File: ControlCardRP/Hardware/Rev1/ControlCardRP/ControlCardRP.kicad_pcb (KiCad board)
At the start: 2 copper layers, 53.5 x 49.5 mm, 46 parts, among them J1 Conn_02x20_Top_Bottom, J2 USB_C_Receptacle_USB2.0_16P, J3 SWD, J4 JST_PK BATTERY, J5 PIN_HEADER BATTERY, SW101 BOOT0, SW102 NRST, U1 AP33772SDKZ-xx-FA02, U101 W25Q128JVS, U102 RP2354B, U103 W25Q128JVS, U2 BQ24075RGT, U3 BQ27427YZFR, U4 MP28167GQ-A-P, Y1 12MHz

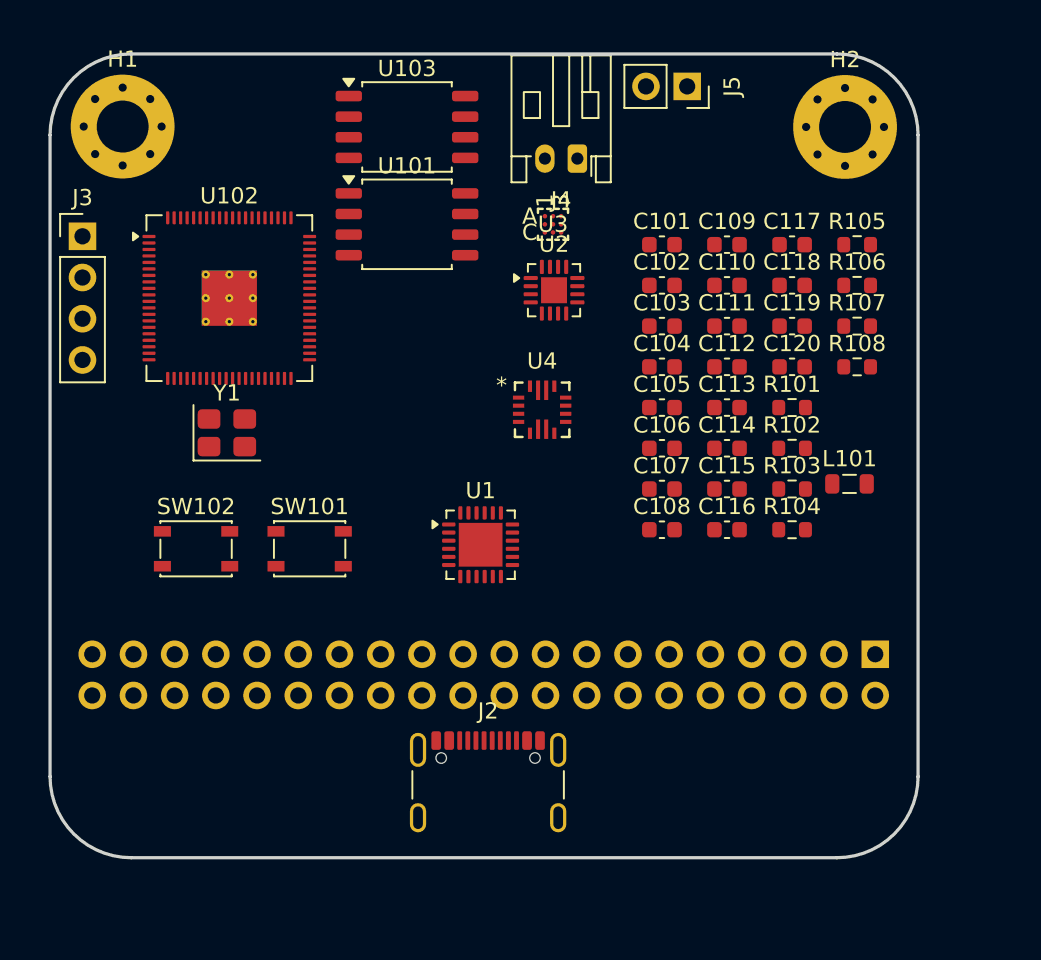
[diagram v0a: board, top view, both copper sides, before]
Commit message: A
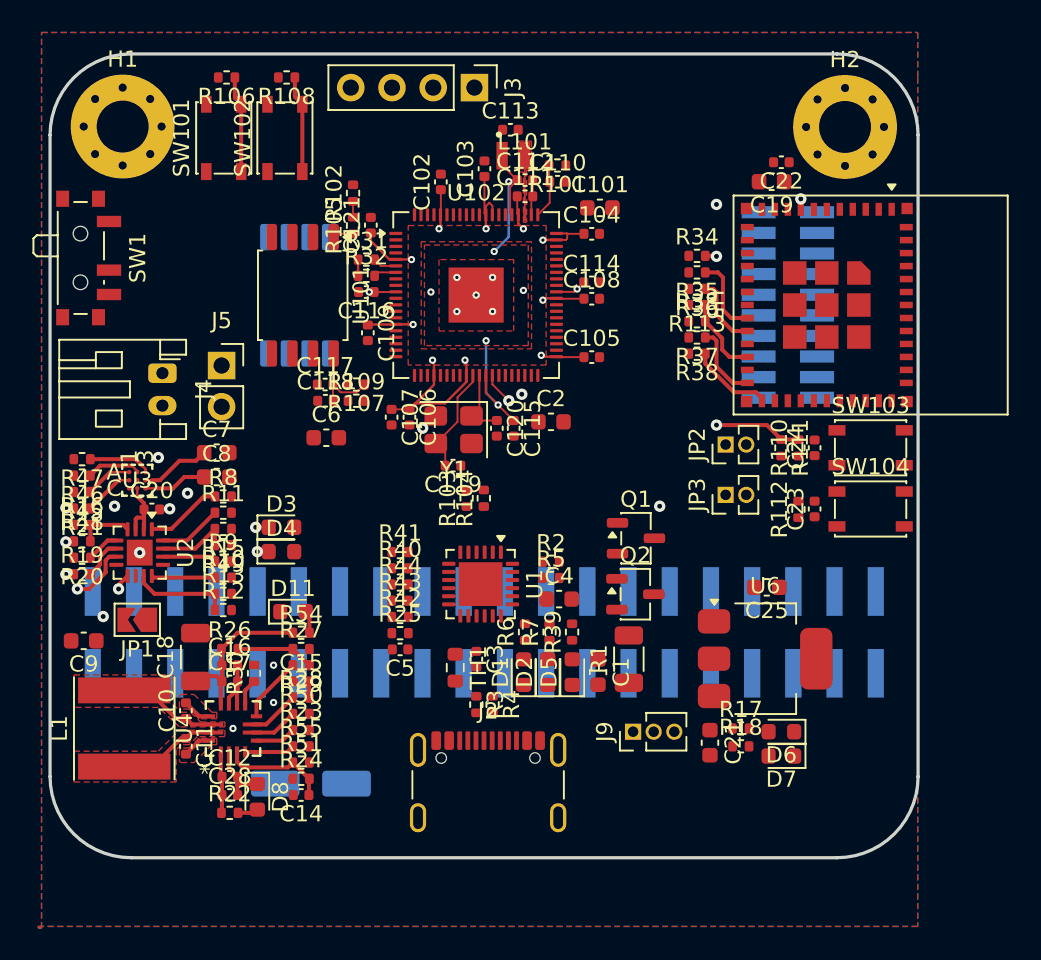
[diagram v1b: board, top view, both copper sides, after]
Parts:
- added C1: 1u, Capacitor_SMD:C_0603_1608Metric, F.Cu at (154.8, 102.6)
- added C10: 100n, Capacitor_SMD:C_0402_1005Metric, F.Cu at (129.4, 105.0)
- added C11: 100n, Capacitor_SMD:C_0402_1005Metric, F.Cu at (129.4, 107.2)
- added C12: 100n, Capacitor_SMD:C_0402_1005Metric, F.Cu at (132.1, 109.1)
- added C121: 100n, Capacitor_SMD:C_0402_1005Metric, F.Cu at (140.8, 75.1)
- added C13: 100u, Capacitor_SMD:CP_Elec_5x5.4, B.Cu at (137.1, 109.5)
- added C14: 22n, Capacitor_SMD:C_0402_1005Metric, F.Cu at (136.5, 110.2)
- added C15: 100n, Capacitor_SMD:C_0402_1005Metric, F.Cu at (136.5, 103.2)
- added C16: 100n, Capacitor_SMD:C_0402_1005Metric, F.Cu at (132.1, 102.2)
- added C17: 100n, Capacitor_SMD:C_0402_1005Metric, F.Cu at (132.1, 103.2)
- added C18: 22u, Capacitor_SMD:C_1206_3216Metric, F.Cu at (130.0, 101.7)
- added C19: 22u, Capacitor_SMD:C_0603_1608Metric, F.Cu at (165.5, 72.4)
- added C2: 10u, Capacitor_SMD:C_0603_1608Metric, F.Cu at (151.9, 87.2)
- added C20: 4u7, Capacitor_SMD:C_0402_1005Metric, F.Cu at (127.3, 92.6)
- added C21: 10u, Capacitor_SMD:C_0603_1608Metric, F.Cu at (161.7, 107.0)
- added C22: 100n, Capacitor_SMD:C_0402_1005Metric, F.Cu at (166.1, 71.2)
- added C23: 100n, Capacitor_SMD:C_0402_1005Metric, F.Cu at (168.1, 92.5)
- added C24: 100n, Capacitor_SMD:C_0402_1005Metric, F.Cu at (168.1, 88.8)
- added C25: 10u, Capacitor_SMD:C_0603_1608Metric, F.Cu at (165.2, 97.4)
- added C28: 10u, Capacitor_SMD:C_0402_1005Metric, F.Cu at (132.1, 110.2)
- added C3: 100n, Capacitor_SMD:C_0402_1005Metric, F.Cu at (147.3, 101.8)
- added C4: 1u, Capacitor_SMD:C_0603_1608Metric, F.Cu at (152.4, 98.1)
- added C5: 100n, Capacitor_SMD:C_0402_1005Metric, F.Cu at (142.6, 101.2)
- added C6: 1u, Capacitor_SMD:C_0603_1608Metric, F.Cu at (138.0, 88.2)
- added C7: 2u2, Capacitor_SMD:C_0603_1608Metric, F.Cu at (131.3, 89.1)
- added C8: 1u, Capacitor_SMD:C_0603_1608Metric, F.Cu at (131.3, 90.6)
- added C9: 10u, Capacitor_SMD:C_0603_1608Metric, F.Cu at (123.1, 100.7)
- added D1: LED, LED_SMD:LED_0603_1608Metric, F.Cu at (150.2, 102.6)
- added D11: LED, LED_SMD:LED_0603_1608Metric, F.Cu at (136.0, 98.9)
- added D2: LED, LED_SMD:LED_0603_1608Metric, F.Cu at (151.7, 102.6)
- added D3: LED, LED_SMD:LED_0603_1608Metric, F.Cu at (135.3, 93.7)
- added D4: LED, LED_SMD:LED_0603_1608Metric, F.Cu at (135.3, 95.2)
- added D5: LED, LED_SMD:LED_0603_1608Metric, F.Cu at (153.2, 102.6)
- added D6: LED, LED_SMD:LED_0603_1608Metric, F.Cu at (166.1, 106.3)
- added D7: LED, LED_SMD:LED_0603_1608Metric, F.Cu at (166.1, 107.8)
- added D8: LED, LED_SMD:LED_0603_1608Metric, F.Cu at (133.8, 110.3)
- added J8: ESP_IO, Connector_PinSocket_1.27mm:PinSocket_2x10_P1.27mm_Vertical_SMD, B.Cu at (166.5, 80.0)
- added J9: Conn_01x03_Pin, Connector_PinHeader_1.27mm:PinHeader_1x03_P1.27mm_Vertical, F.Cu at (156.9, 106.3)
- added JP1: SKIP_BATT, Jumper:SolderJumper-2_P1.3mm_Open_TrianglePad1.0x1.5mm, F.Cu at (126.4, 99.4)
- added JP2: ESP_RXD, Connector_PinHeader_1.27mm:PinHeader_1x02_P1.27mm_Vertical, F.Cu at (162.6, 88.6)
- added JP3: ESP_TXD, Connector_PinHeader_1.27mm:PinHeader_1x02_P1.27mm_Vertical, F.Cu at (162.6, 91.7)
- added L1: 4u7, Inductor_SMD:L_Taiyo-Yuden_NR-60xx, F.Cu at (125.6, 106.1)
- added Q1: NMOS, Package_TO_SOT_SMD:SOT-23-3, F.Cu at (157.1, 94.3)
- added Q2: NMOS, Package_TO_SOT_SMD:SOT-23-3, F.Cu at (157.1, 97.8)
- added R1: 5m, Resistor_SMD:R_1206_3216Metric, F.Cu at (156.7, 101.8)
- added R10: 1k13, Resistor_SMD:R_0402_1005Metric, F.Cu at (131.7, 96.8)
- added R109: 0R, Resistor_SMD:R_0402_1005Metric, F.Cu at (139.9, 85.9)
- added R11: 1k18, Resistor_SMD:R_0402_1005Metric, F.Cu at (131.7, 92.8)
- added R110: 10k, Resistor_SMD:R_0402_1005Metric, F.Cu at (167.1, 88.8)
- added R111: 10k, Resistor_SMD:R_0402_1005Metric, F.Cu at (166.1, 88.8)
- added R112: 10k, Resistor_SMD:R_0402_1005Metric, F.Cu at (167.1, 92.6)
- added R113: 10k, Resistor_SMD:R_0402_1005Metric, F.Cu at (160.9, 80.0)
- added R12: 1k5, Resistor_SMD:R_0402_1005Metric, F.Cu at (131.7, 98.8)
- added R13: 1k5, Resistor_SMD:R_0402_1005Metric, F.Cu at (131.7, 97.8)
- added R15: 0R, Resistor_SMD:R_0402_1005Metric, F.Cu at (131.7, 93.8)
- added R16: 0R, Resistor_SMD:R_0402_1005Metric, F.Cu at (123.0, 93.5)
- added R17: 10k, Resistor_SMD:R_0402_1005Metric, F.Cu at (163.6, 106.1)
- added R18: 10k, Resistor_SMD:R_0402_1005Metric, F.Cu at (163.6, 107.2)
- added R19: 10k, Resistor_SMD:R_0402_1005Metric, F.Cu at (123.0, 96.6)
- added R2: 6k2, Resistor_SMD:R_0402_1005Metric, F.Cu at (151.9, 95.8)
- added R20: 10k, Resistor_SMD:R_0402_1005Metric, F.Cu at (123.0, 95.6)
- added R21: 200k, Resistor_SMD:R_0402_1005Metric, F.Cu at (123.0, 92.5)
- added R22: 10k, Resistor_SMD:R_0402_1005Metric, F.Cu at (132.1, 111.3)
- added R23: 0R, Resistor_SMD:R_0402_1005Metric, F.Cu at (136.5, 106.2)
- added R24: 499k, Resistor_SMD:R_0402_1005Metric, F.Cu at (136.5, 109.2)
- added R25: 100k, Resistor_SMD:R_0402_1005Metric, F.Cu at (142.6, 100.2)
- added R26: 430k, Resistor_SMD:R_0402_1005Metric, F.Cu at (132.1, 101.2)
- added R27: 107k, Resistor_SMD:R_0402_1005Metric, F.Cu at (136.5, 101.2)
- added R28: 499k, Resistor_SMD:R_0402_1005Metric, F.Cu at (136.5, 104.2)
- added R29: 806k, Resistor_SMD:R_0402_1005Metric, F.Cu at (136.5, 102.2)
- added R3: 5k1, Resistor_SMD:R_0402_1005Metric, F.Cu at (147.3, 104.6)
- added R30: 499k, Resistor_SMD:R_0402_1005Metric, F.Cu at (133.6, 102.7)
- added R31: 10k, Resistor_SMD:R_0402_1005Metric, F.Cu at (140.5, 77.2)
- added R32: 10k, Resistor_SMD:R_0402_1005Metric, F.Cu at (140.5, 78.2)
- added R33: 0R, Resistor_SMD:R_0402_1005Metric, F.Cu at (160.9, 81.0)
- added R34: 0R, Resistor_SMD:R_0402_1005Metric, F.Cu at (160.9, 76.9)
- added R35: 0R, Resistor_SMD:R_0402_1005Metric, F.Cu at (160.9, 78.0)
- added R36: 0R, Resistor_SMD:R_0402_1005Metric, F.Cu at (160.9, 79.0)
- added R37: 0R, Resistor_SMD:R_0402_1005Metric, F.Cu at (160.9, 82.0)
- added R38: 0R, Resistor_SMD:R_0402_1005Metric, F.Cu at (160.9, 83.0)
- added R39: 1k, Resistor_SMD:R_0402_1005Metric, F.Cu at (153.2, 100.1)
- added R4: 5k1, Resistor_SMD:R_0402_1005Metric, F.Cu at (148.3, 104.6)
- added R40: 0R, Resistor_SMD:R_0402_1005Metric, F.Cu at (142.6, 96.2)
- added R41: 0R, Resistor_SMD:R_0402_1005Metric, F.Cu at (142.6, 95.2)
- added R42: 0R, Resistor_SMD:R_0402_1005Metric, F.Cu at (142.6, 99.2)
- added R43: 0R, Resistor_SMD:R_0402_1005Metric, F.Cu at (142.6, 98.2)
- added R44: 0R, Resistor_SMD:R_0402_1005Metric, F.Cu at (142.6, 97.2)
- added R45: 0R, Resistor_SMD:R_0402_1005Metric, F.Cu at (123.0, 91.5)
- added R46: 0R, Resistor_SMD:R_0402_1005Metric, F.Cu at (123.0, 90.5)
- added R47: 0R, Resistor_SMD:R_0402_1005Metric, F.Cu at (123.0, 89.5)
- added R48: 10k, Resistor_SMD:R_0402_1005Metric, F.Cu at (123.0, 94.5)
- added R49: 10k, Resistor_SMD:R_0402_1005Metric, F.Cu at (131.7, 94.8)
- added R5: 200R, Resistor_SMD:R_0402_1005Metric, F.Cu at (151.9, 96.8)
- added R50: 0R, Resistor_SMD:R_0402_1005Metric, F.Cu at (136.5, 105.2)
- added R51: 0R, Resistor_SMD:R_0402_1005Metric, F.Cu at (136.5, 108.2)
- added R54: 10k, Resistor_SMD:R_0402_1005Metric, F.Cu at (136.5, 100.2)
- added R55: 0R, Resistor_SMD:R_0402_1005Metric, F.Cu at (136.5, 107.2)
- added R6: 1k, Resistor_SMD:R_0402_1005Metric, F.Cu at (150.3, 100.1)
- added R7: 100k, Resistor_SMD:R_0402_1005Metric, F.Cu at (151.8, 100.1)
- added R8: 10k, Resistor_SMD:R_0402_1005Metric, F.Cu at (131.7, 91.8)
- added R9: R, Resistor_SMD:R_0402_1005Metric, F.Cu at (131.7, 95.8)
- added SW1: SW_SPST, Button_Switch_SMD:SW_SPDT_PCM12, F.Cu at (123.2, 77.1)
- added SW103: NRST, Button_Switch_SMD:SW_SPST_PTS810, F.Cu at (171.6, 88.8)
- added SW104: NRST, Button_Switch_SMD:SW_SPST_PTS810, F.Cu at (171.6, 92.5)
- added TH1: 10k@25C, Resistor_SMD:R_0603_1608Metric, F.Cu at (146.0, 102.3)
- added U5: ESP32-C6-MINI-1, RF_Module:ESP32-C6-MINI-1, F.Cu at (168.9, 80.0)
- added U6: AZ1117-3.3, Package_TO_SOT_SMD:SOT-223-3_TabPin2, F.Cu at (165.1, 101.8)
- C102, C103, C104, C105, C106, C107, C108, C109, C110, C111, C112, C113, C114, C115, C116, C117, C118, C119, C120: footprint Capacitor_SMD:C_0603_1608Metric -> Capacitor_SMD:C_0402_1005Metric
- J1: footprint Connector_PinSocket_2.54mm:PinSocket_2x20_P2.54mm_Vertical -> Connector_PinSocket_2.54mm:PinSocket_2x20_P2.54mm_Vertical_SMD
- L101: footprint Inductor_SMD:L_0805_2012Metric -> footprints:AOTA-B201610S3R3-101-T
- R101, R103, R104, R105: footprint Resistor_SMD:R_0603_1608Metric -> Resistor_SMD:R_0402_1005Metric
- R102, R106, R107, R108: value 1k -> 10k; footprint Resistor_SMD:R_0603_1608Metric -> Resistor_SMD:R_0402_1005Metric
- U102: value RP2354B -> RP2350B; footprint Package_DFN_QFN:QFN-80-1EP_10x10mm_P0.4mm_EP3.4x3.4mm_ThermalVias -> Package_DFN_QFN:QFN-80-1EP_10x10mm_P0.4mm_EP3.4x3.4mm
- U103: moved to B.Cu
- moved R106 40.9 mm to (131.9, 66.0), turned to 180 degrees
- moved R108 39.4 mm to (135.6, 66.0), turned to 180 degrees
- moved J5 33.5 mm to (131.6, 83.7), turned to 0 degrees
- moved R102 31.3 mm to (139.7, 73.1), turned to 90 degrees
- moved R105 31.1 mm to (139.7, 75.1), turned to 90 degrees
- moved R107 31.1 mm to (139.9, 84.9), turned to 180 degrees
- moved U2 30.2 mm to (126.5, 95.2), turned to -90 degrees
- moved U3 30.1 mm to (126.4, 90.8)
- moved C117 30.0 mm to (138.0, 84.9)
- moved C118 29.6 mm to (138.0, 85.9)
- moved J4 28.8 mm to (127.9, 84.2), turned to -90 degrees
- moved U4 27.4 mm to (132.3, 106.1), turned to 90 degrees
- moved L101 27.3 mm to (150.8, 71.8)
- moved C116 26.6 mm to (140.5, 79.2), turned to 180 degrees
- moved SW102 25.9 mm to (135.5, 69.7), turned to 90 degrees
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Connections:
- net BATT_OUT renamed /BATT_OUT
- J1 pad 37: /GPIO36 -> +5V
- J1 pad 38: /GPIO37 -> +5V
- J1 pad 39: /GPIO38 -> GND
- J1 pad 40: /GPIO39 -> GND
- R107 pad 2: /GPIO0 -> Net-(U103-~{CS})
- U1 pad 4: /USB-C PD/UCPD_SDA -> Net-(U1-SDA)
- U1 pad 5: /USB-C PD/UCPD_SCL -> Net-(U1-SCL)
- U1 pad 6: /USB-C PD/UCPD_FLIP -> Net-(U1-FLIP)
- U1 pad 7: /USB-C PD/UCPD_GPIO -> Net-(U1-GPIO)
- U1 pad 8: /USB-C PD/UCPD_LED -> /USB-C PD/LED
- U1 pad 9: /USB-C PD/UCPD_INT -> Net-(U1-INT)
- U102 pad 64: /Controller/VREG_VIN -> +3V3
- U103 pad 1: /GPIO0 -> Net-(U103-~{CS})
- U3 pad A1: /Battery Management/BATT_GPOUT -> Net-(U3-GPOUT)
- U3 pad A2: /Battery Management/BATT_SDA -> Net-(U3-SDA)
- U3 pad A3: /Battery Management/BATT_SCL -> Net-(U3-SCL)
- U3 pad B3: Net-(U3-VDD) -> /Battery Management/VDD
- U4 pad 1: unconnected-(U4-IN-Pad1) -> /GPIO5
- U4 pad 10: unconnected-(U4-AGND-Pad10) -> GND
- U4 pad 11: unconnected-(U4-GND-Pad11) -> GND
- U4 pad 12: unconnected-(U4-OUT-Pad12) -> /Power 5V/OUT
- U4 pad 13: unconnected-(U4-BST2-Pad13) -> Net-(U4-BST2)
- U4 pad 14: unconnected-(U4-SW2-Pad14) -> Net-(U4-SW2)
- U4 pad 15: unconnected-(U4-SW1-Pad15) -> Net-(U4-SW1)
- U4 pad 16: unconnected-(U4-BST1-Pad16) -> Net-(U4-BST1)
- U4 pad 2: unconnected-(U4-GND-Pad2) -> GND
- U4 pad 3: unconnected-(U4-EN-Pad3) -> /Power 5V/EN
- U4 pad 4: unconnected-(U4-ALT-Pad4) -> /Power 5V/ALT
- U4 pad 5: unconnected-(U4-SCL-Pad5) -> /Power 5V/SCL
- U4 pad 6: unconnected-(U4-SDA-Pad6) -> /Power 5V/SDA
- U4 pad 7: unconnected-(U4-OC-Pad7) -> /Power 5V/OC
- U4 pad 8: unconnected-(U4-FB-Pad8) -> /Power 5V/FB
- U4 pad 9: unconnected-(U4-VCC-Pad9) -> /Power 5V/VCC
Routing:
- net +3V3: track 0.00 -> 41.3 mm, vias 0 -> 10
- net +1V1: track 0.00 -> 28.0 mm, vias 0 -> 8
- net /ESP32-C6 Wireless Co-Processor/EN: track 0.00 -> 25.7 mm, vias 0 -> 4
- net /Controller/SWCLK: track 0.00 -> 24.3 mm, vias 0 -> 1
- net /Controller/SWDIO: track 0.00 -> 21.3 mm, vias 0 -> 1
- net /Battery Management/~{PGOOD}: track 0.00 -> 17.6 mm, vias 0 -> 2
- net GND: track 0.00 -> 14.7 mm, vias 0 -> 19
- net /Battery Management/~{CHG}: track 0.00 -> 11.2 mm, vias 0 -> 2
- net /Power 5V/OUT: track 0.00 -> 10.2 mm
- net /Power 5V/EN: track 0.00 -> 6.76 mm
- net /Controller/XIN: track 0.00 -> 6.75 mm
- net Net-(U4-SW2): track 0.00 -> 6.37 mm
- net Net-(U4-SW1): track 0.00 -> 6.37 mm
- net /BATT_OUT: track 0.00 -> 6.10 mm
- net Net-(R108-Pad1): track 0.00 -> 5.99 mm
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- added copper zone on F.Cu, net +1V1
- added copper zone on F.Cu, net +3V3
- added copper zone on F.Cu, net /Controller/VREG_LX
- added copper zone on B.Cu, net GND
- added copper zone on F.Cu, net GND
- added copper zone on In1.Cu, net GND
- added copper zone on In2.Cu, net GND
- added copper zone on F.Cu, net Net-(U4-BST1)
- added copper zone on F.Cu, net Net-(U4-BST2)
- added copper zone on F.Cu, net Net-(U4-SW1)
- added copper zone on F.Cu, net Net-(U4-SW2)
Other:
- copper layers 2 -> 4
